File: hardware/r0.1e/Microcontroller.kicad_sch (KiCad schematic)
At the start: 100 parts, among them J10 UART, J2 USB_C, J3 OLED, J8 +12V, J9 STLink, SW1 Button Up, SW2 Button Down, SW3 Reset, SW4 Button Escape, SW5 Button Left, SW6 Button Enter, SW7 Button Right, U10 STM32F405RGTx, U11 TPS73233, U2 TP6841S6, U3 USBLC6-2, U4 W25Q16, X1 12 MHz TCXO, Y1 8 MHz, Y2 32 kHz

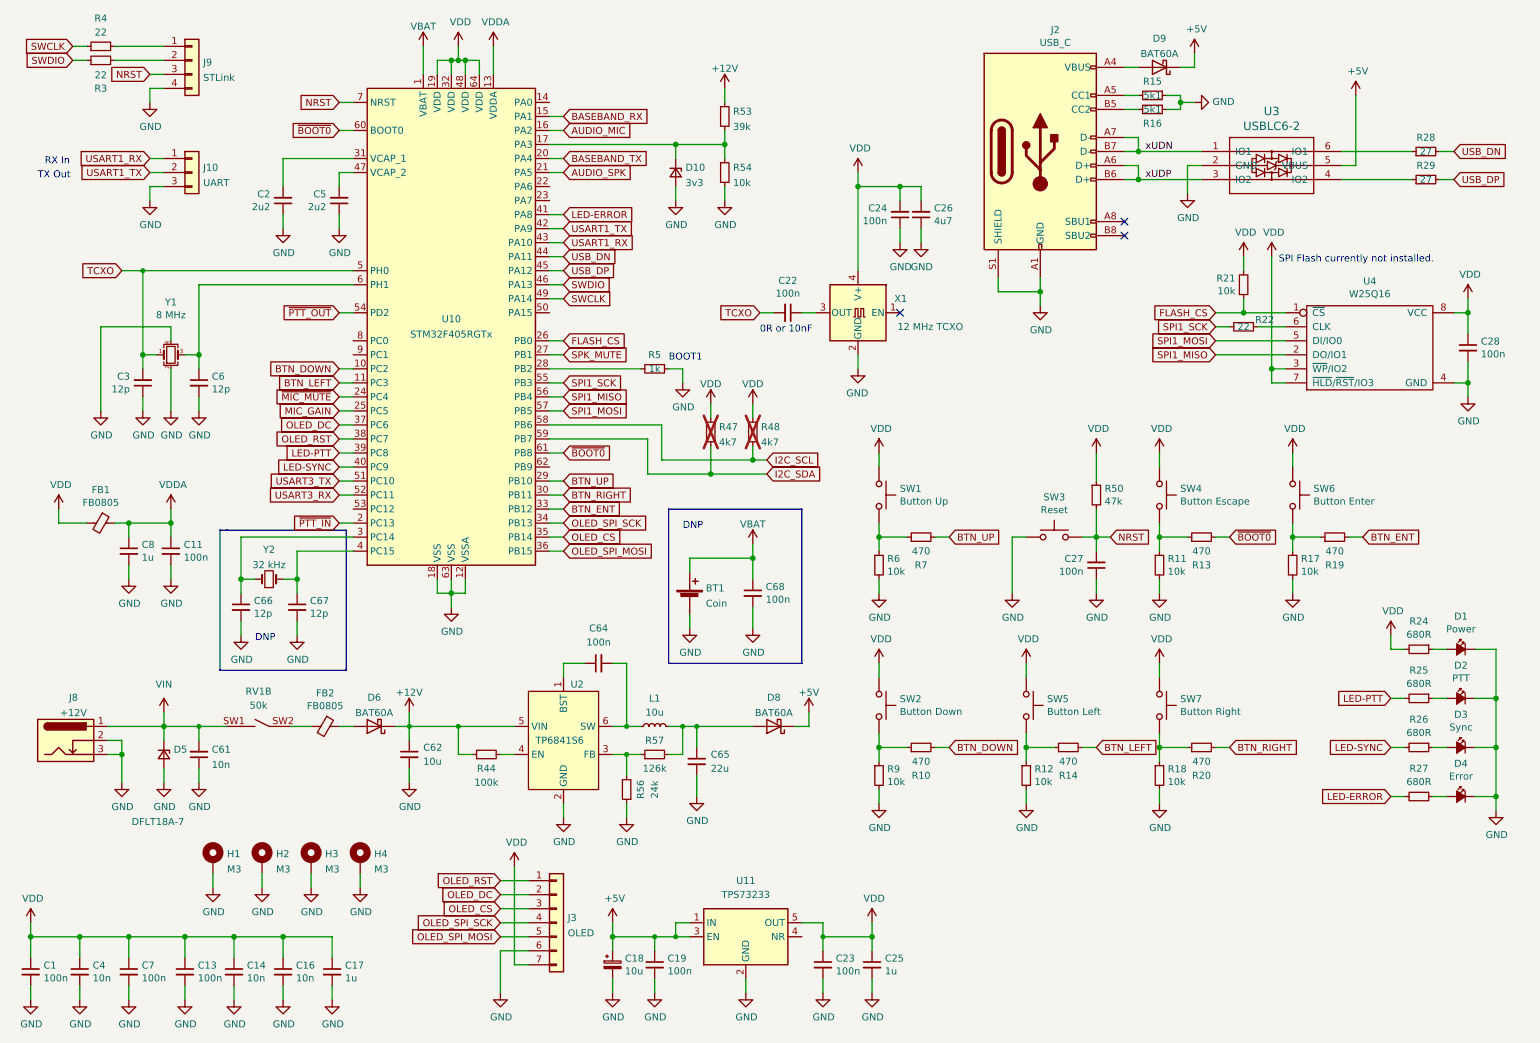
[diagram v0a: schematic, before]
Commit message: WIP r0.1e power switch
👀
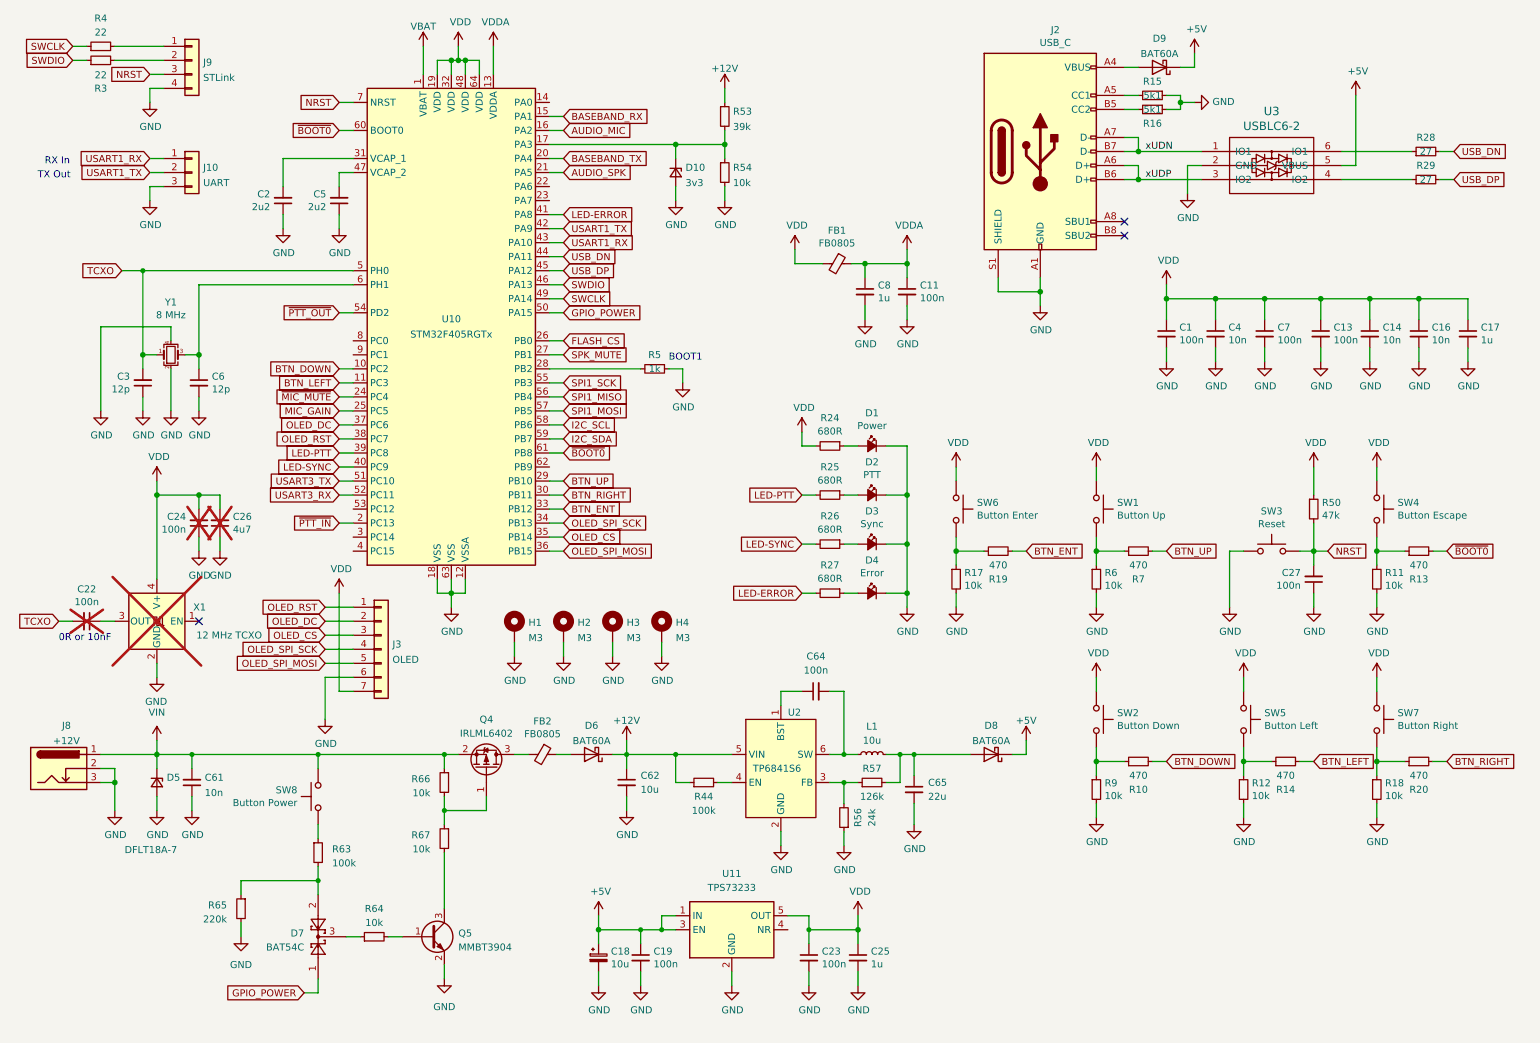
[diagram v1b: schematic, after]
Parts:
- removed BT1: Coin, Battery:BatteryHolder_Keystone_3000_1x12mm, symbol Device:Battery_Cell
- removed C28, C68: 100n, pkl_dipol:C_0603, symbol pkl_device:pkl_C_Small
- removed C66, C67: 12p, pkl_dipol:C_0603, symbol pkl_device:pkl_C_Small
- removed R21: 10k, pkl_dipol:R_0603, symbol pkl_device:pkl_R_Small
- removed R22: 22, pkl_dipol:R_0603, symbol pkl_device:pkl_R_Small
- removed R47, R48: 4k7, pkl_dipol:R_0603, symbol pkl_device:pkl_R_Small
- removed RV1: 50k, M17-SmartMic:PTR901, symbol M17-SmartMic:R_Potentiometer_Switch
- removed U4: W25Q16, Package_SO:SOIC-8_3.9x4.9mm_P1.27mm, symbol pkl_memory:W25Q
- removed Y2: 32 kHz, Crystal:Crystal_SMD_MicroCrystal_CC8V-T1A-2Pin_2.0x1.2mm, symbol Device:Crystal_Small
- added D7: BAT54C, Package_TO_SOT_SMD:SOT-23, symbol Diode:BAT54C
- added Q4: IRLML6402, Package_TO_SOT_SMD:SOT-23, symbol Transistor_FET:IRLML6402
- added Q5: MMBT3904, Package_TO_SOT_SMD:SOT-23, symbol Transistor_BJT:MMBT3904
- added R63: 100k, symbol Device:R_Small
- added R64, R66, R67: 10k, symbol Device:R_Small
- added R65: 220k, symbol Device:R_Small
- added SW8: Button Power, pkl_buttons_switches:SW_SPST_PTS645, symbol Switch:SW_Push
- C22, C24, C26, X1: now not fitted
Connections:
- net GND: now also Q5.2 (E), R65.2
- net VIN: now also Q4.2 (S), R66.1, SW8.1
- net at FB2.2: now also Q4.3 (D)
- net GPIO_POWER: now reaches U10.50 (PA15)
- net GPIO_POWER: now also D7.1
- new net: D7.3, R64.1
- new net: Q5.1 (B), R64.2
- new net: Q4.1 (G), R66.2, R67.1
- new net: Q5.3 (C), R67.2
- new net: D7.2, R63.2, R65.1
- new net: R63.1, SW8.2
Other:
- note removed: "DNP"
- note removed: "SPI Flash currently not installed."
- moved on the sheet: C1, C11, C13, C14, C16, C17, C18, C19, C23, C25, C27, C4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
